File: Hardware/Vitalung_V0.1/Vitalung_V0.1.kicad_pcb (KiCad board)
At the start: 2 copper layers, 82.2 x 36 mm, 54 parts, among them J1 Conn_01x06, Q1 FS8205A, Q2 AO3400A, Q3 AO3401A, SW1 SW_SPDT, U1 ESP32C3_Seeed-Studio, U10 MT3608, U2 DW01A, U3 TP5100, U4 AMS1117-3.3

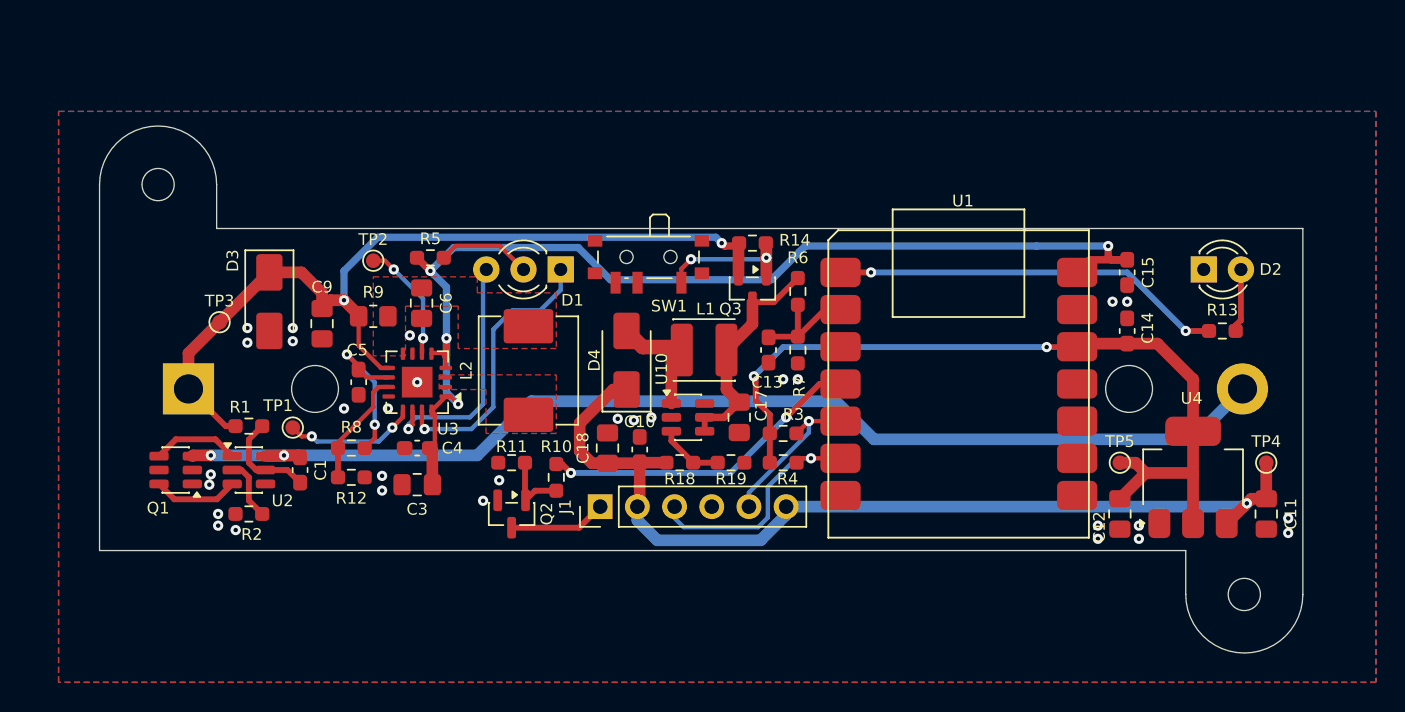
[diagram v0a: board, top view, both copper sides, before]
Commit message: PCB DXF change
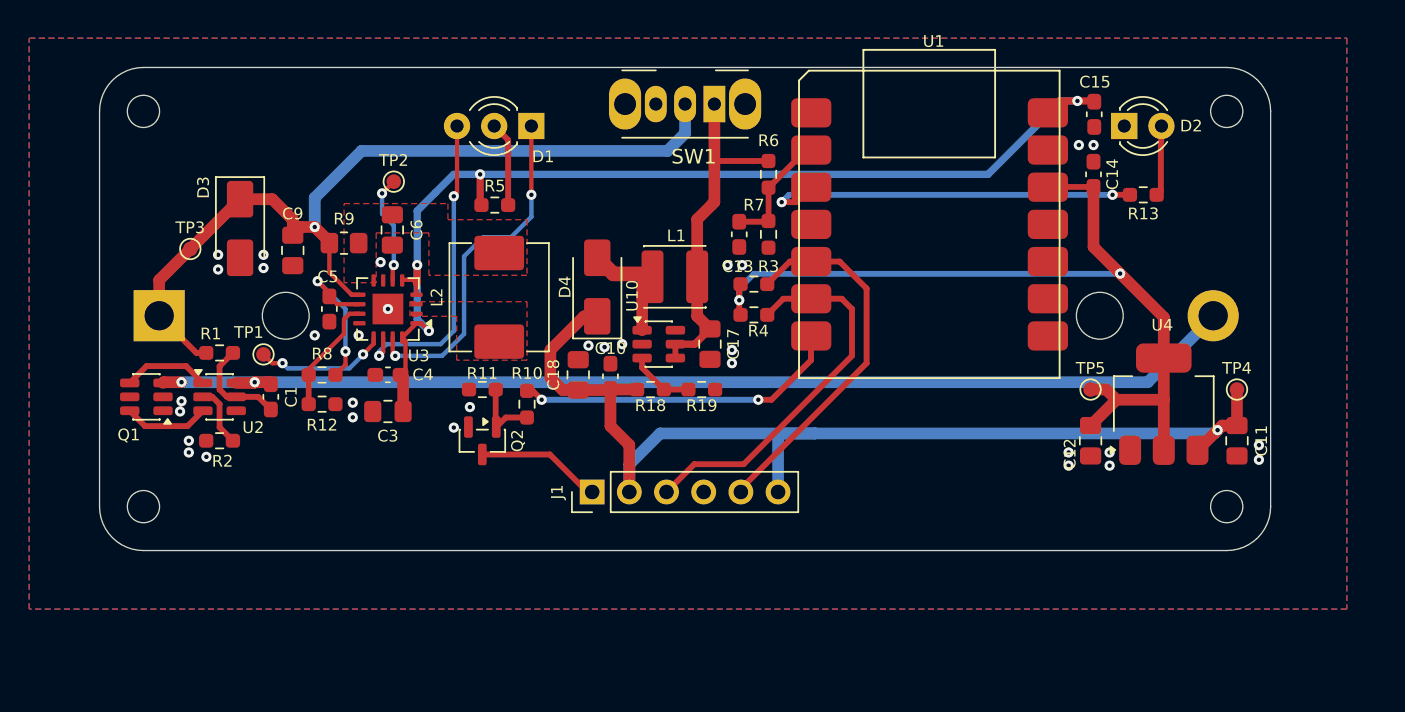
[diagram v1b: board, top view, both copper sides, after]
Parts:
- removed Q3: AO3401A, Package_TO_SOT_SMD:SOT-23
- removed R14: 100K, Resistor_SMD:R_0603_1608Metric_Pad0.98x0.95mm_HandSolder
- added H3: MountingHole, MountingHole:MountingHole_2.2mm_M2, F.Cu at (120.8, 107.0)
- added H4: MountingHole, MountingHole:MountingHole_2.2mm_M2, F.Cu at (194.8, 80.0)
- SW1: footprint Button_Switch_SMD:SW_SPDT_PCM12 -> Button_Switch_THT:SW_Slide_SPDT_Angled_CK_OS102011MA1Q
- moved SW1 11.7 mm to (159.8, 79.5)
- moved D2 11.2 mm to (187.8, 81.0)
- moved U1 11.1 mm to (165.6, 98.2)
- moved C15 11.0 mm to (185.8, 80.2)
- moved C14 10.9 mm to (185.7, 84.3)
- moved R13 10.8 mm to (189.1, 85.7)
- moved R3 10.4 mm to (162.5, 91.8)
- moved R4 10.3 mm to (162.5, 93.9)
- moved D1 10.0 mm to (147.3, 81.0)
- moved R6 8.25 mm to (163.5, 84.3)
- moved C13 8.15 mm to (161.5, 88.4)
- moved R7 8.15 mm to (163.5, 88.4)
- moved H2 6.12 mm to (194.8, 107.0)
- moved R5 5.69 mm to (144.8, 86.4)
- moved TP2 5.58 mm to (137.9, 84.8)
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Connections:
- C17 pad 1: Net-(Q3-D) -> Net-(SW1-A)
- L1 pad 1: Net-(Q3-D) -> Net-(SW1-A)
- R13 pad 1: Net-(U1-PA02_A0_D0) -> Net-(U1-PA10_A2_D2)
- R6 pad 2: Net-(Q3-D) -> Net-(SW1-A)
- SW1 pad 1: Net-(Q3-G) -> Net-(SW1-A)
- SW1 pad 2: GND -> +BATT
- U1 pad 1: Net-(U1-PA02_A0_D0) -> unconnected-(U1-PA02_A0_D0-Pad1)
- U1 pad 3: unconnected-(U1-PA10_A2_D2-Pad3) -> Net-(U1-PA10_A2_D2)
- U1 pad 4: Heater_En -> unconnected-(U1-PA11_A3_D3-Pad4)
- U1 pad 7: unconnected-(U1-PB08_A6_D6_TX-Pad7) -> Heater_En
- U10 pad 4: Net-(Q3-D) -> Net-(SW1-A)
- U10 pad 5: Net-(Q3-D) -> Net-(SW1-A)
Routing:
- net Net-(U1-PA02_A0_D0): track 26.8 -> 0.00 mm, vias 2 -> 0
- net Net-(U1-PA10_A2_D2): track 0.00 -> 26.4 mm, vias 0 -> 2
- net Net-(SW1-A): track 0.00 -> 23.7 mm
- net Net-(Q3-D): track 15.4 -> 0.00 mm
- net SDA: track 10.9 -> 25.6 mm, vias 1 -> 0
- net SCL: track 16.7 -> 26.3 mm, vias 1 -> 0
- net +5V: track 65.8 -> 75.3 mm
- net Net-(Q3-G): track 9.24 -> 0.00 mm, vias 2 -> 0
- net Net-(D1-K2): track 16.6 -> 21.4 mm, vias 1 -> 2
- net Net-(D1-K1): track 19.2 -> 24.0 mm, vias 1 -> 2
- net +3V3: track 55.9 -> 60.3 mm
- net VBUS: track 76.8 -> 73.4 mm
- net Net-(BT1--): track 78.3 -> 76.1 mm
- net Net-(J1-Pin_1): track 6.65 -> 8.56 mm
- net +BATT: track 60.1 -> 58.8 mm, vias 2 -> 1
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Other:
- board size 82.2 x 36 mm -> 80 x 33 mm
